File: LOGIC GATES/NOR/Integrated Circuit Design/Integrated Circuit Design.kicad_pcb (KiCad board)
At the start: 2 copper layers, 25 x 40 mm, 0 parts

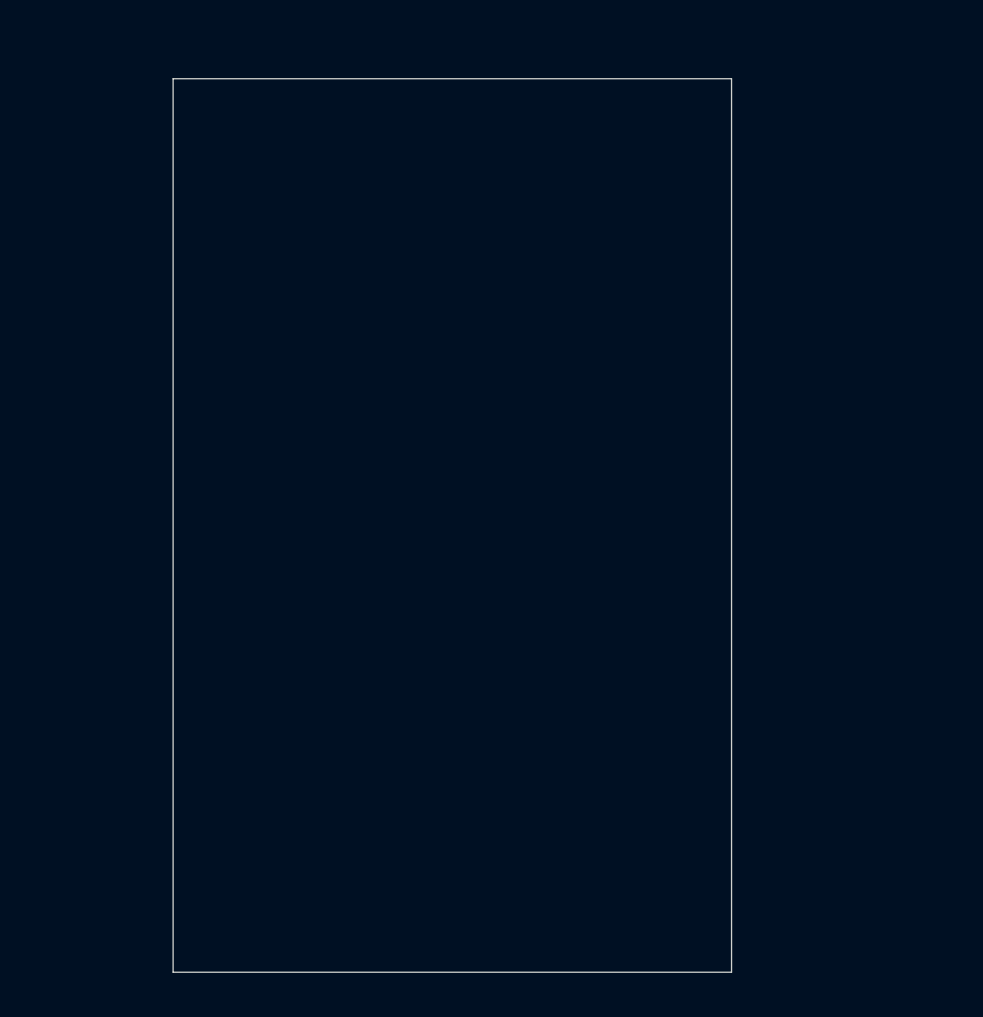
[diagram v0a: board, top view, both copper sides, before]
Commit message: Auto-update: 22.12.2025 16:16:21,18
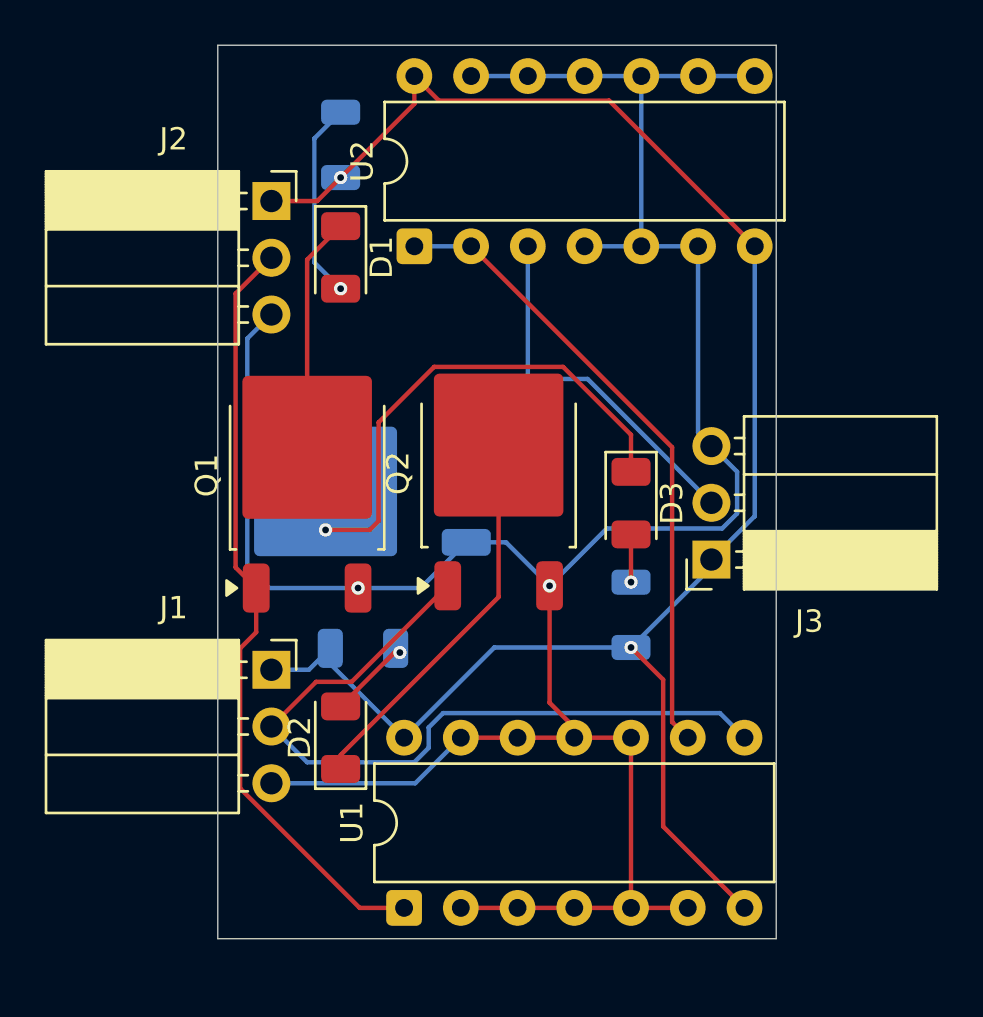
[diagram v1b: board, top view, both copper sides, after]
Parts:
- added D1: LED, LED_SMD:LED_1206_3216Metric, F.Cu at (115.5, 84.5)
- added D2: LED, LED_SMD:LED_1206_3216Metric, F.Cu at (115.5, 106.0)
- added D3: LED, LED_SMD:LED_1206_3216Metric, F.Cu at (128.5, 95.5)
- added J1: Conn_01x03_Socket, Connector_PinSocket_2.54mm:PinSocket_1x03_P2.54mm_Horizontal, F.Cu at (112.4, 103.0)
- added J2: Conn_01x03_Socket, Connector_PinSocket_2.54mm:PinSocket_1x03_P2.54mm_Horizontal, F.Cu at (112.4, 82.0)
- added J3: Conn_01x03_Socket, Connector_PinSocket_2.54mm:PinSocket_1x03_P2.54mm_Horizontal, F.Cu at (132.1, 98.0)
- added Q1: QM6006D, Package_TO_SOT_SMD:TO-252-2, F.Cu at (114.0, 94.3)
- added Q2: QM6006D, Package_TO_SOT_SMD:TO-252-2, F.Cu at (122.6, 94.2)
- added Q3: QM6006D, Package_TO_SOT_SMD:TO-252-2, B.Cu at (116.1, 95.0)
- added R1: R, Resistor_SMD:R_1206_3216Metric, B.Cu at (115.5, 79.5)
- added R2: R, Resistor_SMD:R_1206_3216Metric, B.Cu at (116.5, 102.0)
- added R3: R, Resistor_SMD:R_1206_3216Metric, B.Cu at (128.5, 100.5)
- added U1: 4075, Package_DIP:DIP-14_W7.62mm, F.Cu at (118.3, 113.6)
- added U2: 4011, Package_DIP:DIP-14_W7.62mm, F.Cu at (118.8, 84.0)
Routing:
- net Net-(J1-Pin_3): track 0.00 -> 117.3 mm, vias 0 -> 2
- net Net-(J1-Pin_1): track 0.00 -> 82.1 mm, vias 0 -> 2
- net Net-(J2-Pin_2): track 0.00 -> 34.7 mm
- net Net-(J1-Pin_2): track 0.00 -> 34.2 mm
- net Net-(U1-Pad9): track 0.00 -> 28.6 mm
- net Net-(D3-K): track 0.00 -> 22.2 mm, vias 0 -> 1
- net Net-(J3-Pin_2): track 0.00 -> 20.4 mm
- net Net-(D2-K): track 0.00 -> 17.4 mm
- net Net-(D1-K): track 0.00 -> 10.5 mm
- net Net-(D1-A): track 0.00 -> 8.87 mm, vias 0 -> 1
- net Net-(D2-A): track 0.00 -> 3.65 mm, vias 0 -> 1
- net Net-(D3-A): track 0.00 -> 2.14 mm, vias 0 -> 1
